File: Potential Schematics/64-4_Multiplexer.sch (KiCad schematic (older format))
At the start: 0 parts

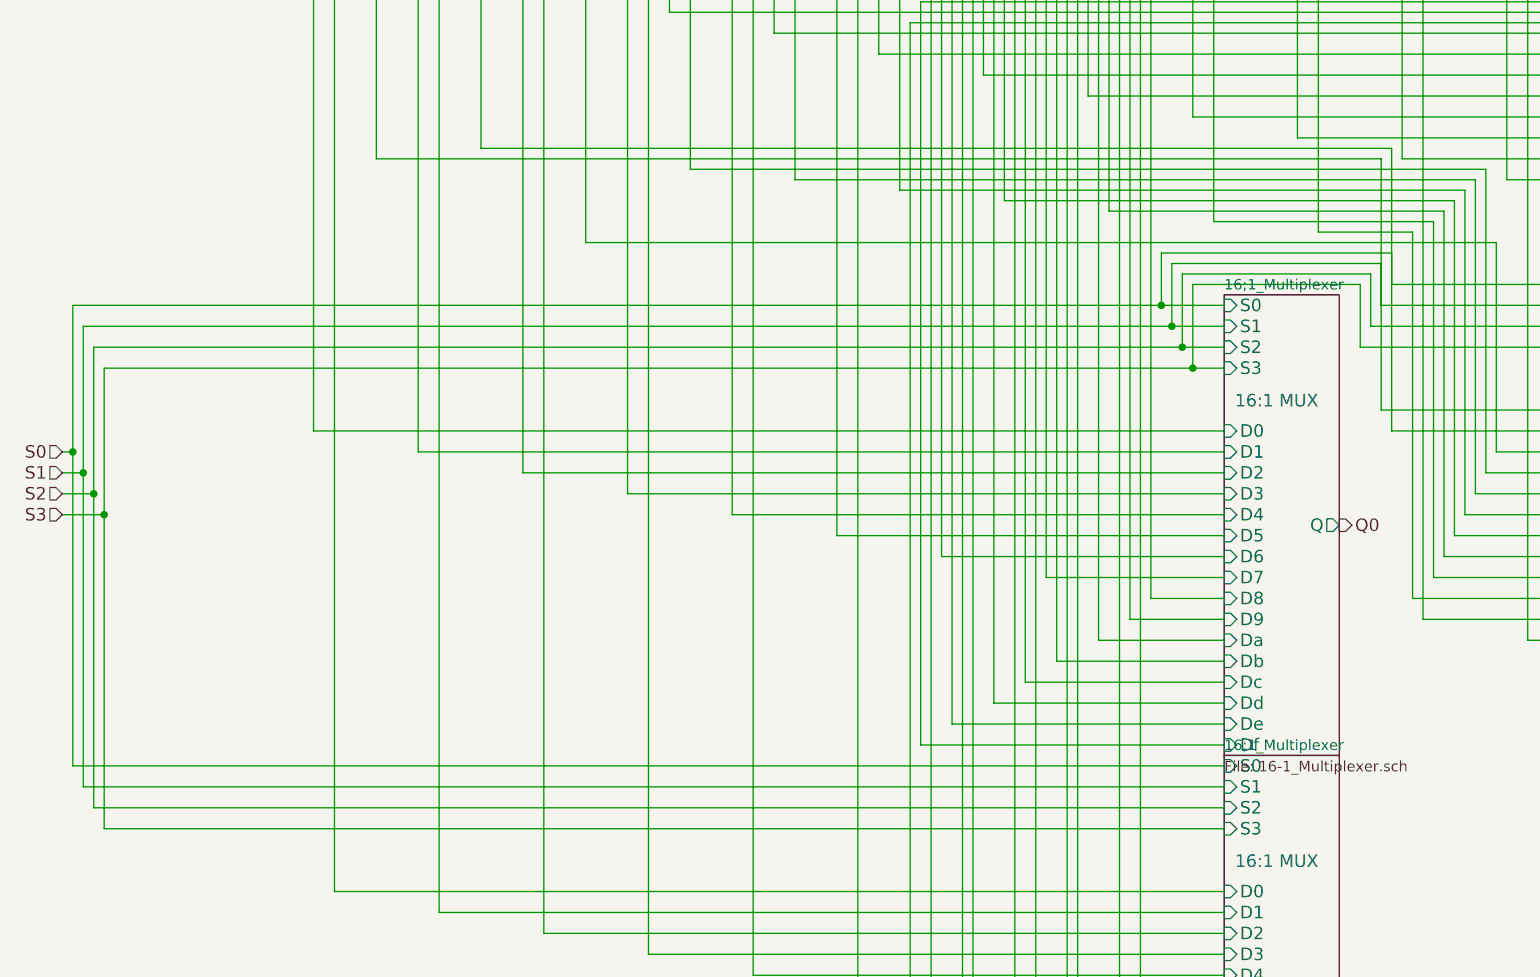
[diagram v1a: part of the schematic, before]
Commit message: Finished PCB
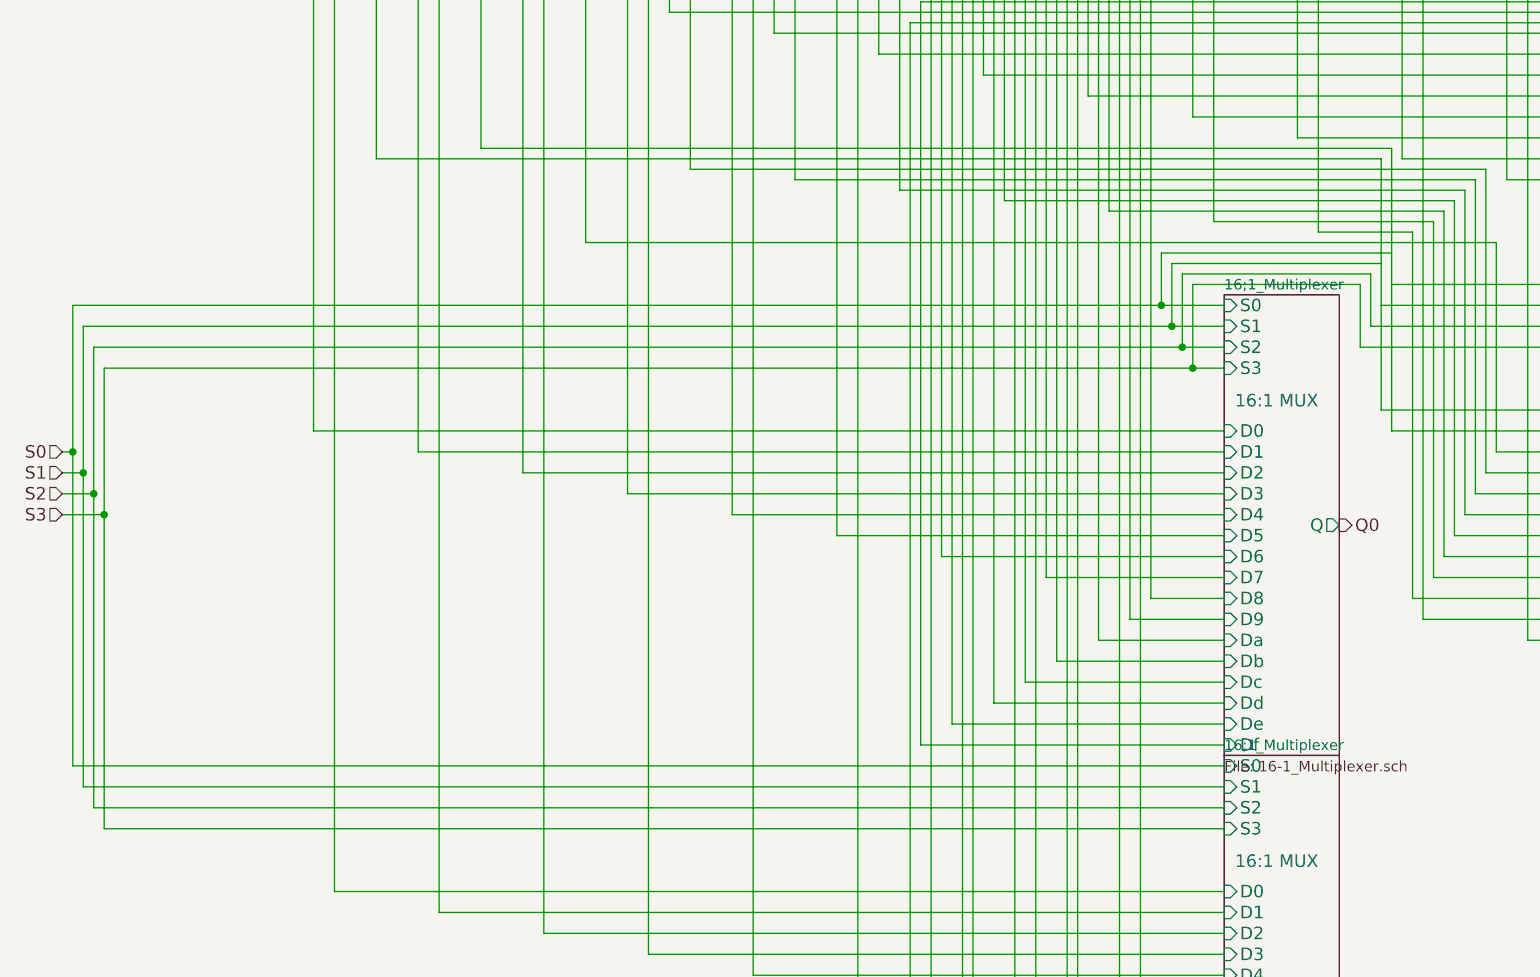
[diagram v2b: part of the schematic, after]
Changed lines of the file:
@@
 $Descr A4 11693 8268
 encoding utf-8
-Sheet 377 451
+Sheet 377 456
 Title "64:4 Multiplexer"
 Date "2018-09-14"
@@
 	850  3900 900  3900
 Wire Wire Line
-	900  3200 900  5400
-Wire Wire Line
-	900  3200 6400 3200
-Wire Wire Line
-	6400 3300 950  3300
-Wire Wire Line
-	950  3300 950  5500
+	900  3200 900  3900
+Wire Wire Line
+	900  3200 6100 3200
+Wire Wire Line
+	6400 3300 6150 3300
+Wire Wire Line
+	950  3300 950  4000
 Wire Wire Line
 	950  4000 850  4000
@@
 	850  4100 1000 4100
 Wire Wire Line
-	1000 3400 1000 5600
-Wire Wire Line
-	1000 3400 6400 3400
-Wire Wire Line
-	6400 3500 1050 3500
-Wire Wire Line
-	1050 3500 1050 5700
+	1000 3400 1000 4100
+Wire Wire Line
+	1000 3400 6200 3400
+Wire Wire Line
+	6400 3500 6250 3500
+Wire Wire Line
+	1050 3500 1050 4200
 Wire Wire Line
 	1050 4200 850  4200
@@
 	6150 3000 7150 3000
 Wire Wire Line
-	7150 3000 7150 3200
-Wire Wire Line
 	7150 3200 10000 3200
 Connection ~ 6150 3300
@@
 	10000 3100 7200 3100
 Wire Wire Line
-	7200 3100 7200 2950
-Wire Wire Line
 	7200 2950 6100 2950
 Wire Wire Line
@@
 	10000 3800 7200 3800
 Wire Wire Line
-	7200 3800 7200 2450
-Wire Wire Line
 	7200 2450 2850 2450
 Wire Wire Line
@@
 Wire Wire Line
 	10000 3700 7150 3700
-Wire Wire Line
-	7150 3700 7150 2500
 Wire Wire Line
 	7150 2500 2350 2500
@@
 Text Notes 10450 1400 2    60   ~ 0
 16:1 MUX\n
+Wire Wire Line
+	900  3900 900  5400
+Wire Wire Line
+	950  4000 950  5500
+Wire Wire Line
+	1000 4100 1000 5600
+Wire Wire Line
+	1050 4200 1050 5700
+Wire Wire Line
+	6250 3500 1050 3500
+Wire Wire Line
+	6200 3400 6400 3400
+Wire Wire Line
+	6150 3300 950  3300
+Wire Wire Line
+	6100 3200 6400 3200
+Wire Wire Line
+	7150 2500 7150 3700
+Wire Wire Line
+	7200 2450 7200 3800
 $EndSCHEMATC
